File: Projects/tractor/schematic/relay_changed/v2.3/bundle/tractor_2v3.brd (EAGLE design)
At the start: 66.5 x 45.5 mm, 80 parts, among them IC1 PIC16F1824, IC2 33063A, K2 RL703, Q1 IRLML2402, Q2 IRLML2402, Q3 IRLML2402, T1 BC547

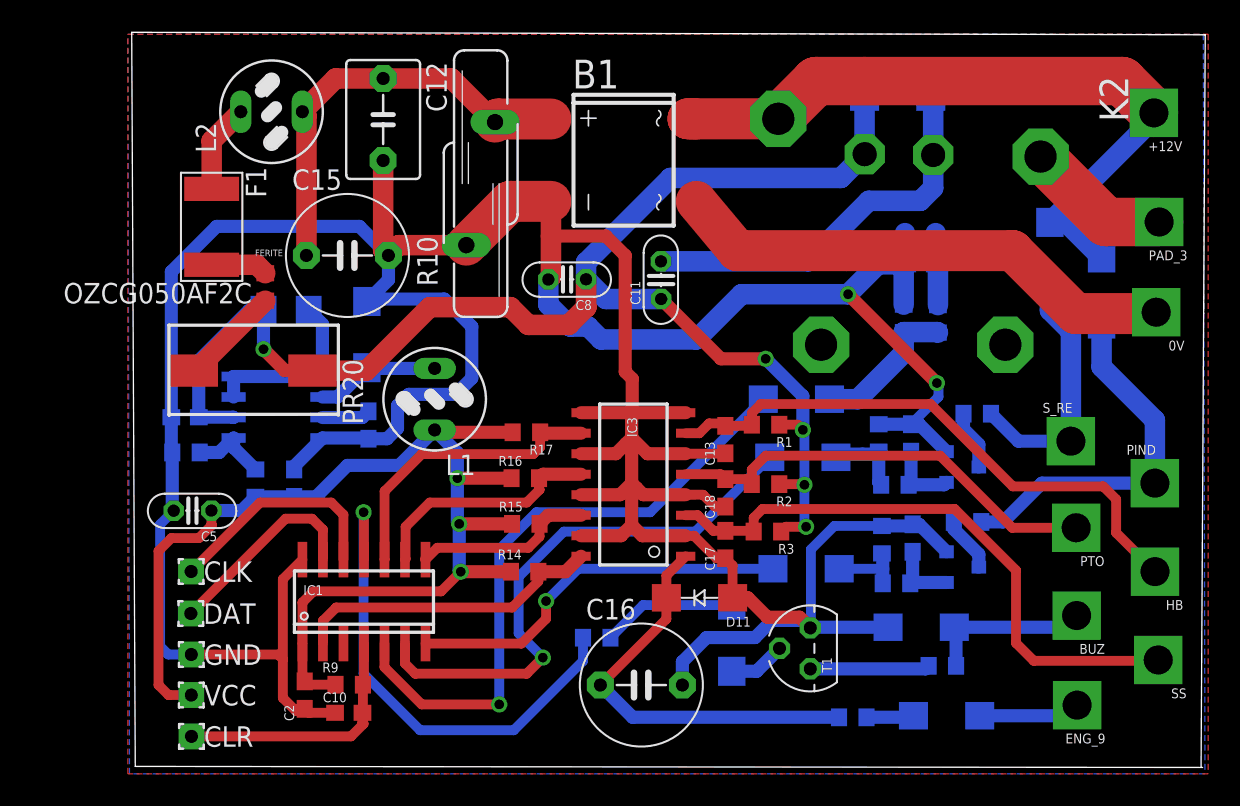
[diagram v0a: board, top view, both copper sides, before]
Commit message: folder structure updated
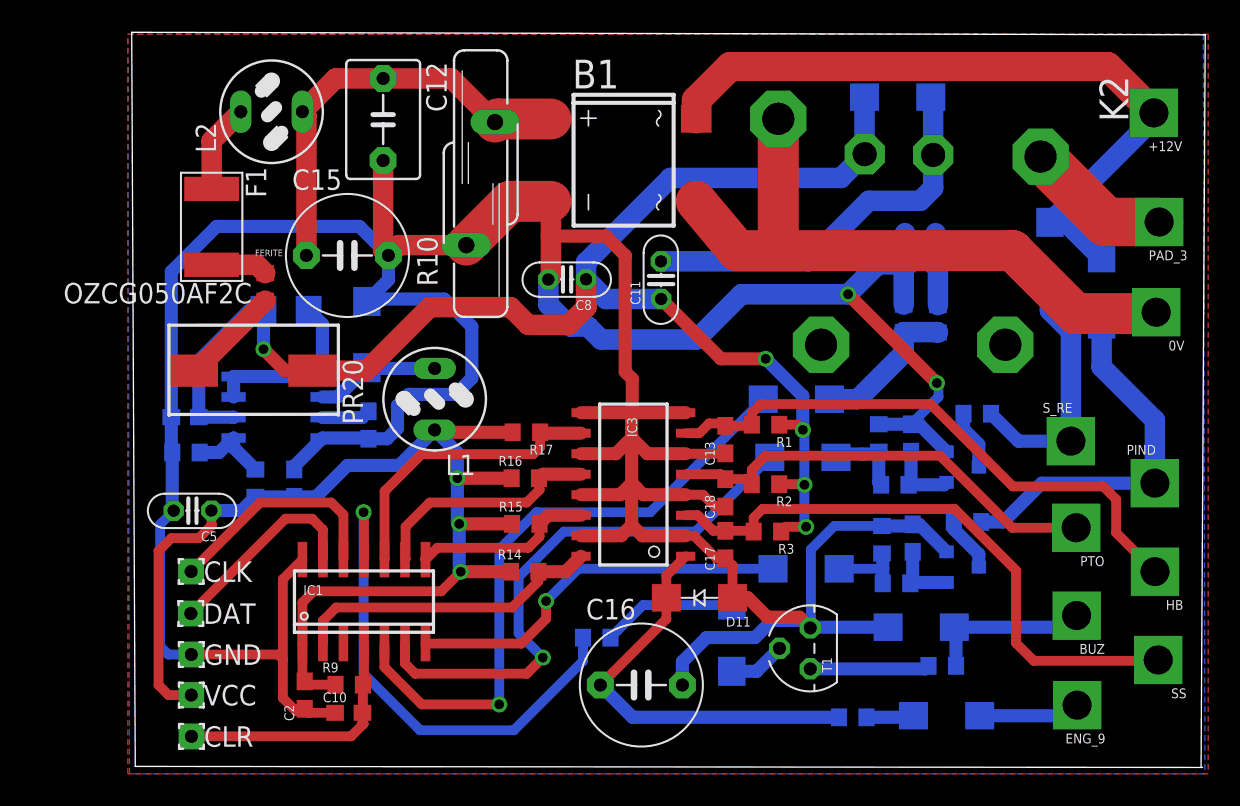
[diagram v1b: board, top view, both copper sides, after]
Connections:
- net 12V_8: no longer K2.NO
- net N$1: now also K2.NO
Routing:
- net N$1: track 31.6 -> 39.9 mm
